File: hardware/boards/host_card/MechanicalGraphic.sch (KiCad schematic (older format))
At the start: 7 parts

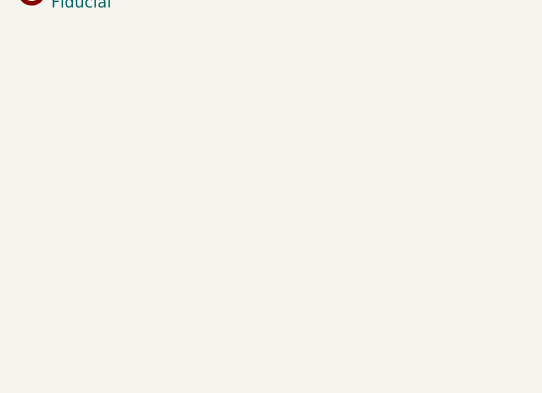
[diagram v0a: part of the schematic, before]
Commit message: More fiddling with the DM stuff
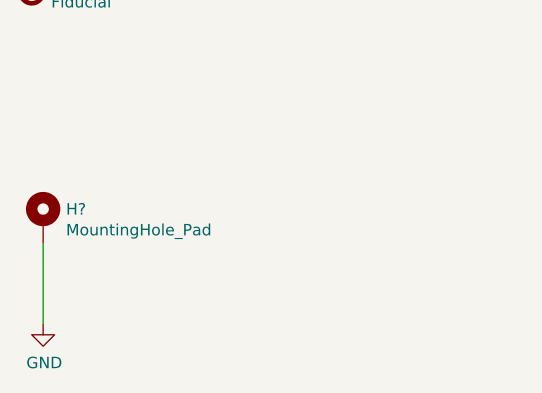
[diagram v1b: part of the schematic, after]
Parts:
- added H?: MountingHole_Pad, MountingHole:MountingHole_3.2mm_M3_Pad_Via, symbol Mechanical:MountingHole_Pad
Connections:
- new net GND: H?.1
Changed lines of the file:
@@
 	1    0    0    -1
 $EndComp
+$Comp
+L Mechanical:MountingHole_Pad H?
+U 1 1 5EEC9E4D
+P 1650 3750
+F 0 "H?" H 1750 3799 50  0000 L CNN
+F 1 "MountingHole_Pad" H 1750 3708 50  0000 L CNN
+F 2 "MountingHole:MountingHole_3.2mm_M3_Pad_Via" H 1650 3750 50  0001 C CNN
+F 3 "~" H 1650 3750 50  0001 C CNN
+	1    1650 3750
+	1    0    0    -1
+$EndComp
+$Comp
+L power:GND #PWR?
+U 1 1 5EECB465
+P 1650 4200
+F 0 "#PWR?" H 1650 3950 50  0001 C CNN
+F 1 "GND" H 1655 4027 50  0000 C CNN
+F 2 "" H 1650 4200 50  0001 C CNN
+F 3 "" H 1650 4200 50  0001 C CNN
+	1    1650 4200
+	1    0    0    -1
+$EndComp
+Wire Wire Line
+	1650 3850 1650 4200
 $EndSCHEMATC
